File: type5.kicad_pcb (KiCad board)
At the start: 2 copper layers, 80 x 50 mm, 3 parts, among them P1 CONN_01X09, P2 CONN_01X26, U1 TEENSYPP2

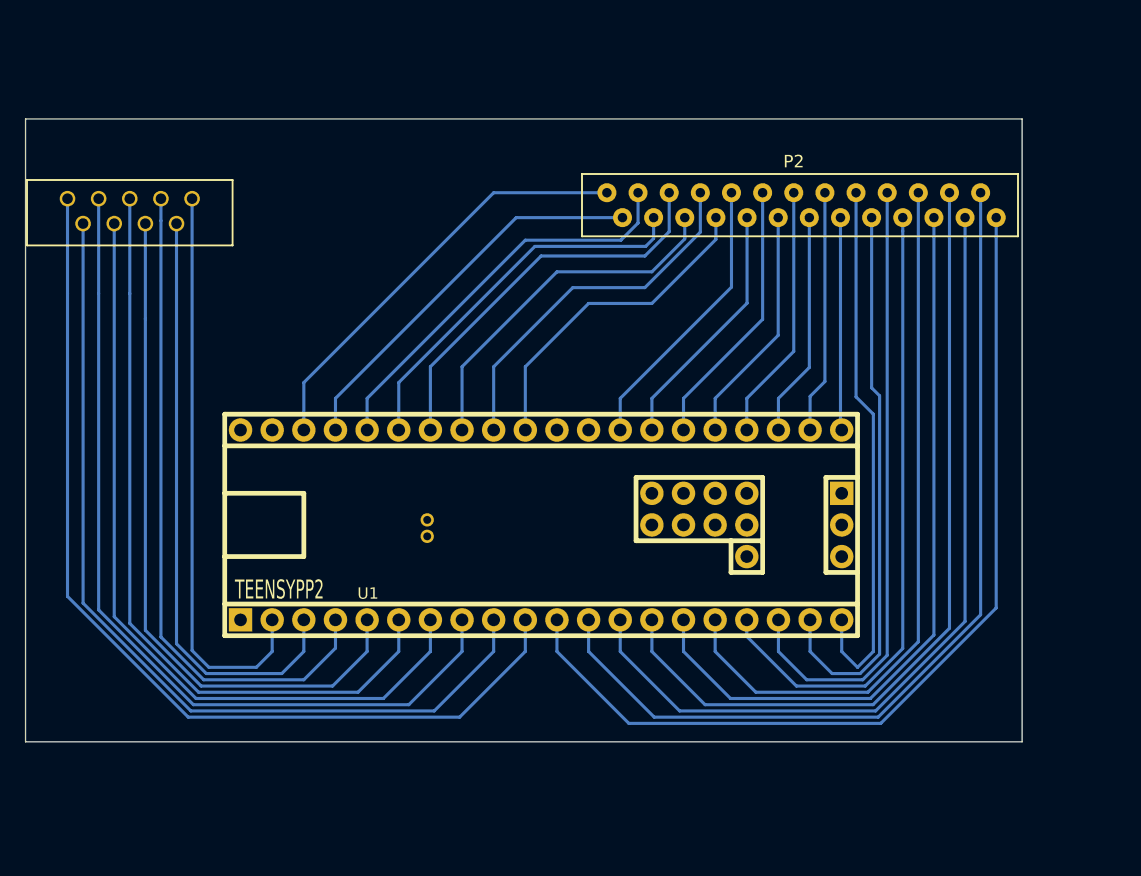
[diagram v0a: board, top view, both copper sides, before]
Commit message: pcb mod
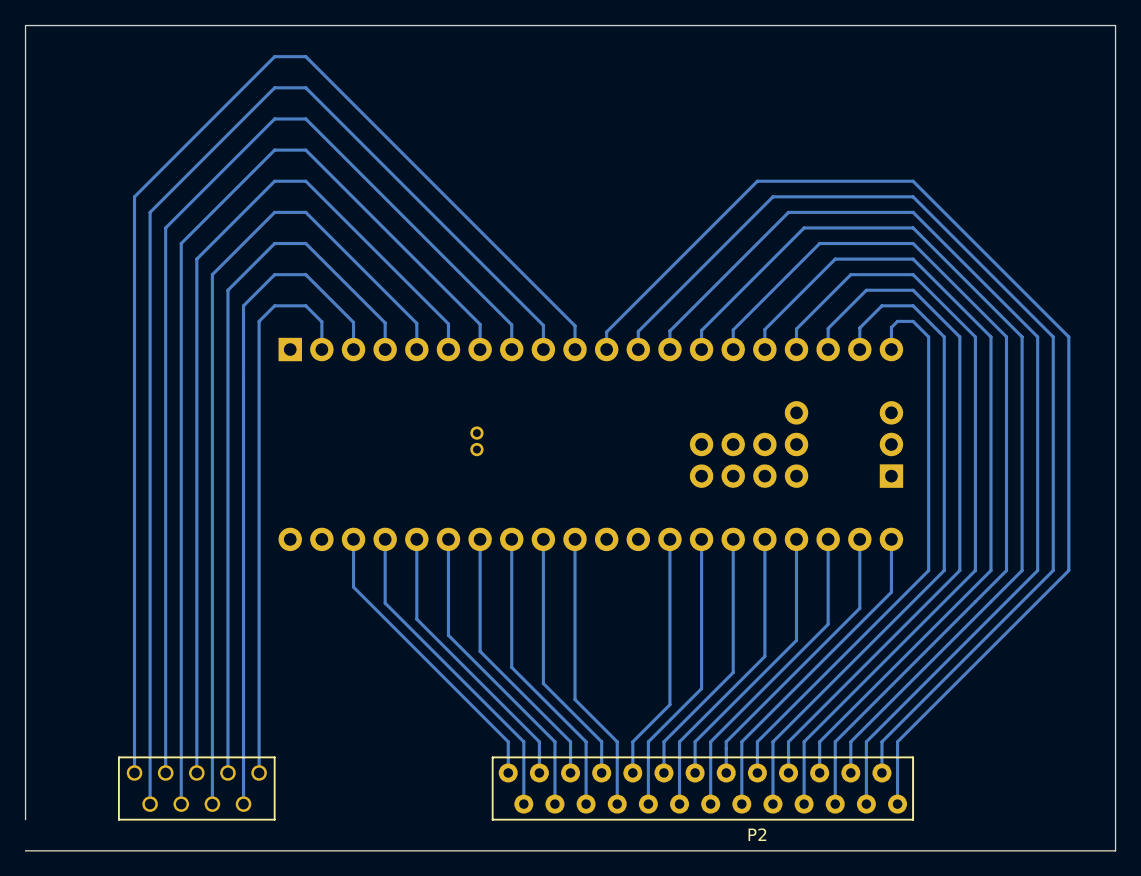
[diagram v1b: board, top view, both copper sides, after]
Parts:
- U1: moved to B.Cu
- moved P2 48.0 mm to (153.8, 120.0)
- moved P1 46.9 mm to (113.8, 121.2)
- moved U1 7.59 mm to (145.4, 96.1)
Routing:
- net Net-(P1-Pad2): track 71.5 -> 93.1 mm
- net Net-(P1-Pad1): track 77.4 -> 97.1 mm
- net Net-(P2-Pad26): track 75.4 -> 91.9 mm
- net Net-(P1-Pad4): track 63.8 -> 79.9 mm
- net Net-(P2-Pad24): track 67.6 -> 82.3 mm
- net Net-(P1-Pad3): track 69.6 -> 84.0 mm
- net Net-(P2-Pad22): track 59.8 -> 72.7 mm
- net Net-(P2-Pad20): track 51.3 -> 63.1 mm
- net Net-(P2-Pad25): track 73.5 -> 84.6 mm
- net Net-(P1-Pad6): track 56.0 -> 66.8 mm
- net Net-(P2-Pad1): track 34.5 -> 23.9 mm
- net Net-(P2-Pad5): track 31.9 -> 21.8 mm
- net Net-(P2-Pad3): track 32.6 -> 22.8 mm
- net Net-(P2-Pad23): track 65.7 -> 75.0 mm
- net Net-(P2-Pad16): track 17.1 -> 26.2 mm
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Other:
- board size 80 x 50 mm -> 87.5 x 66.2 mm
